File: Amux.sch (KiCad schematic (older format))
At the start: 3 parts, among them U16 74LVC32, U6 74LVC257, U7 74LVC257

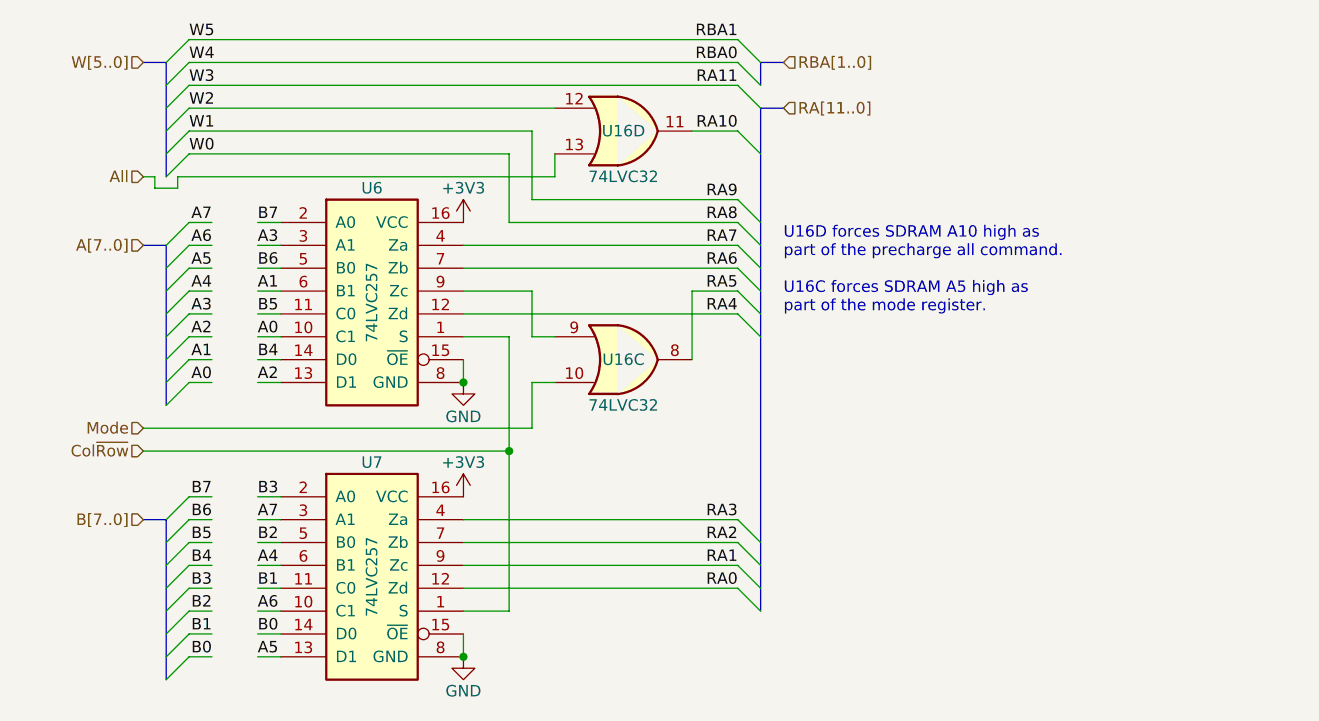
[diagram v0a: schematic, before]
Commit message: PAL
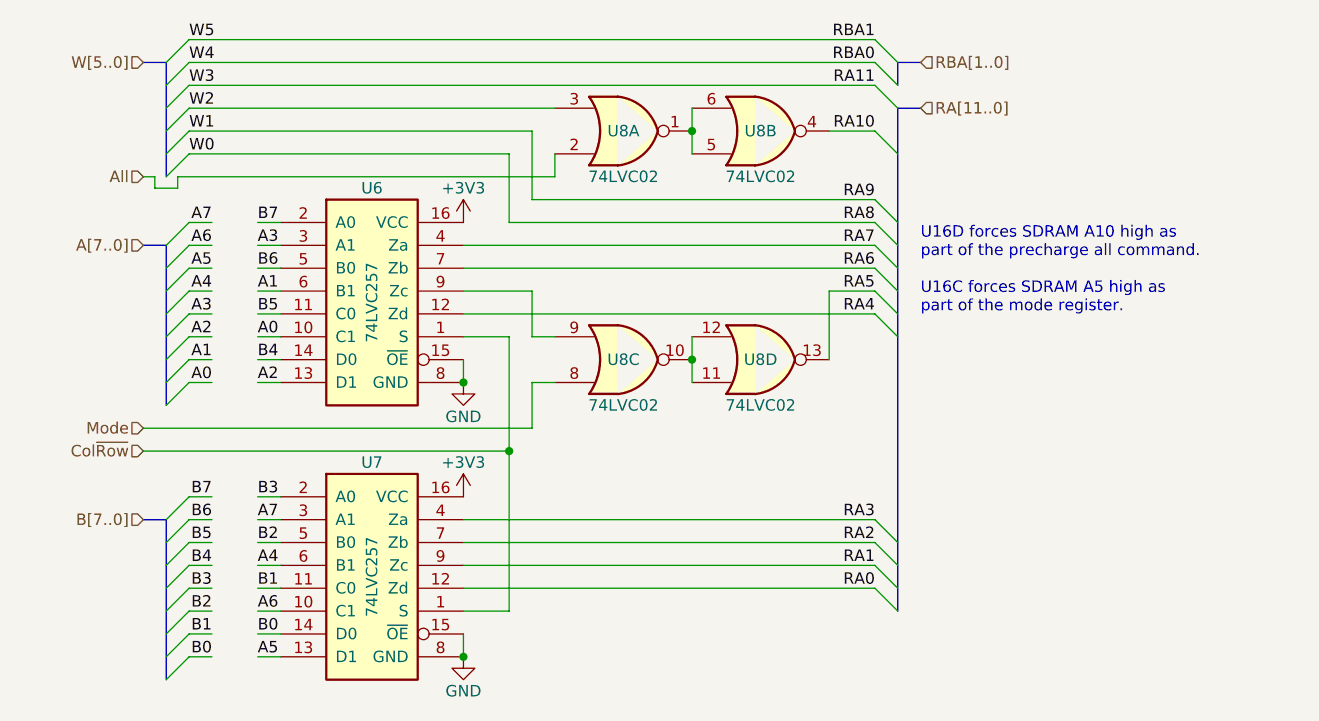
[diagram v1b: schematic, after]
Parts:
- removed U16: 74LVC32, stdpads:TSSOP-14_4.4x5mm_P0.65mm, symbol 74xx:74LS32
- added U8: 74LVC02, stdpads:TSSOP-14_4.4x5mm_P0.65mm, symbol 74xx:74LS02
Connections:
- net All: now also U8.2
- net Mode: now also U8.8
- net RA10: now also U8.4
- net RA5: now also U8.13
- net W2: now also U8.3
- net at U6.9 (Zc): now also U8.9
- new net: U8.10, U8.11, U8.12
- new net: U8.1, U8.5, U8.6
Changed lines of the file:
@@
 $Descr USLetter 11000 8500
 encoding utf-8
-Sheet 6 6
+Sheet 3 5
 Title ""
 Date ""
@@
 $EndComp
 Connection ~ 5500 5450
-Text Label 6700 5150 2    50   ~ 0
-RA0
-Text Label 6700 5050 2    50   ~ 0
-RA1
-Text Label 6700 4950 2    50   ~ 0
-RA2
-Text Label 6700 4850 2    50   ~ 0
-RA3
 Text Label 4600 4050 0    50   ~ 0
 A0
@@
 Text Label 4600 4850 0    50   ~ 0
 A7
-Text Label 6700 3650 2    50   ~ 0
-RA7
-Text Label 6700 3750 2    50   ~ 0
-RA6
-Text Label 6700 3950 2    50   ~ 0
-RA4
 Text Label 4600 5350 0    50   ~ 0
 B0
@@
 Text Label 4600 3550 0    50   ~ 0
 B7
-Text Label 6700 3550 2    50   ~ 0
-RA8
-Text Label 6700 3450 2    50   ~ 0
-RA9
 Text Label 4300 3250 0    50   ~ 0
 W0
 Text Label 4300 3150 0    50   ~ 0
 W1
-Text Label 6700 3150 2    50   ~ 0
-RA10
-Text Label 6700 2950 2    50   ~ 0
-RA11
 Text Label 4300 3050 0    50   ~ 0
 W2
 Text Label 4300 2950 0    50   ~ 0
 W3
-Text Label 6700 2850 2    50   ~ 0
-RBA0
 Text Label 4300 2850 0    50   ~ 0
 W4
@@
 Wire Wire Line
 	5700 4550 5700 5250
-Wire Wire Line
-	6700 5150 5500 5150
-Wire Wire Line
-	5500 5050 6700 5050
-Wire Wire Line
-	6700 4950 5500 4950
-Wire Wire Line
-	5500 4850 6700 4850
-Wire Wire Line
-	6700 3950 5500 3950
-Wire Wire Line
-	5500 3750 6700 3750
-$Comp
-L 74xx:74LS32 U?
-U 4 1 6061EDB0
-P 6200 3150
-AR Path="/CF1C1573/6061EDB0" Ref="U?"  Part="1"
-AR Path="/6061EDB0" Ref="U?"  Part="1"
-AR Path="/6060D166/6061EDB0" Ref="U16"  Part="4"
-F 0 "U16" H 6200 3150 50  0000 C CNN
-F 1 "74LVC32" H 6200 2950 50  0000 C CNN
-F 2 "stdpads:TSSOP-14_4.4x5mm_P0.65mm" H 6200 3150 50  0001 C CNN
-F 3 "http://www.ti.com/lit/gpn/sn74ls02" H 6200 3150 50  0001 C CNN
-	4    6200 3150
-	1    0    0    -1
-$EndComp
-Wire Wire Line
-	5700 3550 6700 3550
-Wire Wire Line
-	6700 3450 5800 3450
 Wire Wire Line
 	5700 3250 5700 3550
@@
 	1    0    0    -1
 $EndComp
-Wire Wire Line
-	5500 3650 6700 3650
-Wire Wire Line
-	6700 3150 6500 3150
-Wire Wire Line
-	6700 3850 6500 3850
-$Comp
-L 74xx:74LS32 U?
-U 3 1 6061EDE7
-P 6200 4150
-AR Path="/CF1C1573/6061EDE7" Ref="U?"  Part="1"
-AR Path="/6061EDE7" Ref="U?"  Part="1"
-AR Path="/6060D166/6061EDE7" Ref="U16"  Part="3"
-F 0 "U16" H 6200 4150 50  0000 C CNN
-F 1 "74LVC32" H 6200 3950 50  0000 C CNN
-F 2 "stdpads:TSSOP-14_4.4x5mm_P0.65mm" H 6200 4150 50  0001 C CNN
-F 3 "http://www.ti.com/lit/gpn/sn74ls02" H 6200 4150 50  0001 C CNN
-	3    6200 4150
-	1    0    0    -1
-$EndComp
-Wire Wire Line
-	6500 3850 6500 4150
-Text Label 6700 2750 2    50   ~ 0
-RBA1
 Text HLabel 4100 2850 0    50   Input ~ 0
 W[5..0]
@@
 	4100 2850 4200 2850
 Wire Wire Line
-	4300 2750 6700 2750
-Wire Wire Line
-	4300 2850 6700 2850
-Wire Wire Line
-	4300 2950 6700 2950
+	4300 2750 7300 2750
+Wire Wire Line
+	4300 2850 7300 2850
 Wire Wire Line
 	4300 3050 5900 3050
@@
 Wire Wire Line
 	4250 3350 5900 3350
-Text HLabel 6900 2850 2    50   Input ~ 0
+Text HLabel 7500 2850 2    50   Input ~ 0
 RBA[1..0]
 Entry Wire Line
-	6800 2950 6700 2850
-Entry Wire Line
-	6800 2850 6700 2750
-Wire Bus Line
-	6900 2850 6800 2850
-Wire Bus Line
-	6800 2850 6800 2950
-Entry Wire Line
-	6800 3250 6700 3150
-Entry Wire Line
-	6800 3050 6700 2950
-Wire Bus Line
-	6900 3050 6800 3050
-Text HLabel 6900 3050 2    50   Input ~ 0
+	7400 2950 7300 2850
+Entry Wire Line
+	7400 2850 7300 2750
+Wire Bus Line
+	7500 2850 7400 2850
+Wire Bus Line
+	7400 2850 7400 2950
+Wire Bus Line
+	7500 3050 7400 3050
+Text HLabel 7500 3050 2    50   Input ~ 0
 RA[11..0]
-Entry Wire Line
-	6800 3650 6700 3550
-Entry Wire Line
-	6800 3550 6700 3450
-Entry Wire Line
-	6800 3750 6700 3650
-Entry Wire Line
-	6800 3950 6700 3850
-Entry Wire Line
-	6800 3850 6700 3750
-Entry Wire Line
-	6800 4050 6700 3950
-Entry Wire Line
-	6800 5050 6700 4950
-Entry Wire Line
-	6800 4950 6700 4850
-Entry Wire Line
-	6800 5150 6700 5050
-Entry Wire Line
-	6800 5250 6700 5150
 Wire Wire Line
 	4250 3400 4250 3350
@@
 Wire Wire Line
 	5800 4250 5800 4450
-Text Notes 6900 3950 0    50   ~ 0
+Text Notes 7500 3950 0    50   ~ 0
 U16D forces SDRAM A10 high as\npart of the precharge all command.\n\nU16C forces SDRAM A5 high as\npart of the mode register.
-Text Label 6700 3850 2    50   ~ 0
+Wire Wire Line
+	7300 5150 5500 5150
+Wire Wire Line
+	5500 5050 7300 5050
+Wire Wire Line
+	5500 4850 7300 4850
+Wire Wire Line
+	7300 4950 5500 4950
+Wire Wire Line
+	7300 3950 5500 3950
+Wire Wire Line
+	5500 3750 7300 3750
+Wire Wire Line
+	7300 3850 7100 3850
+Wire Wire Line
+	5500 3650 7300 3650
+Wire Wire Line
+	7300 3450 5800 3450
+Wire Wire Line
+	5700 3550 7300 3550
+Wire Wire Line
+	4300 2950 7300 2950
+Entry Wire Line
+	7400 5250 7300 5150
+Entry Wire Line
+	7400 5150 7300 5050
+Entry Wire Line
+	7400 4950 7300 4850
+Entry Wire Line
+	7400 5050 7300 4950
+Entry Wire Line
+	7400 4050 7300 3950
+Entry Wire Line
+	7400 3850 7300 3750
+Entry Wire Line
+	7400 3950 7300 3850
+Entry Wire Line
+	7400 3750 7300 3650
+Entry Wire Line
+	7400 3550 7300 3450
+Entry Wire Line
+	7400 3650 7300 3550
+Entry Wire Line
+	7400 3050 7300 2950
+Entry Wire Line
+	7400 3250 7300 3150
+Text Label 7300 3850 2    50   ~ 0
 RA5
+Text Label 7300 2750 2    50   ~ 0
+RBA1
+Text Label 7300 2850 2    50   ~ 0
+RBA0
+Text Label 7300 2950 2    50   ~ 0
+RA11
+Text Label 7300 3150 2    50   ~ 0
+RA10
+Text Label 7300 3450 2    50   ~ 0
+RA9
+Text Label 7300 3550 2    50   ~ 0
+RA8
+Text Label 7300 3950 2    50   ~ 0
+RA4
+Text Label 7300 3750 2    50   ~ 0
+RA6
+Text Label 7300 3650 2    50   ~ 0
+RA7
+Text Label 7300 4850 2    50   ~ 0
+RA3
+Text Label 7300 4950 2    50   ~ 0
+RA2
+Text Label 7300 5050 2    50   ~ 0
+RA1
+Text Label 7300 5150 2    50   ~ 0
+RA0
+$Comp
+L 74xx:74LS02 U?
+U 3 1 64E55E47
+P 6200 4150
+AR Path="/606ED367/64E55E47" Ref="U?"  Part="1"
+AR Path="/64E55E47" Ref="U?"  Part="1"
+AR Path="/6060D166/64E55E47" Ref="U8"  Part="3"
+F 0 "U8" H 6200 4150 50  0000 C CNN
+F 1 "74LVC02" H 6200 4350 50  0000 C CNN
+F 2 "stdpads:TSSOP-14_4.4x5mm_P0.65mm" H 6200 4150 50  0001 C CNN
+F 3 "http://www.ti.com/lit/gpn/sn74LS08" H 6200 4150 50  0001 C CNN
+	3    6200 4150
+	1    0    0    1
+$EndComp
+$Comp
+L 74xx:74LS02 U?
+U 4 1 64E60EEF
+P 6800 4150
+AR Path="/606ED367/64E60EEF" Ref="U?"  Part="1"
+AR Path="/64E60EEF" Ref="U?"  Part="1"
+AR Path="/6060D166/64E60EEF" Ref="U8"  Part="4"
+F 0 "U8" H 6800 4150 50  0000 C CNN
+F 1 "74LVC02" H 6800 4350 50  0000 C CNN
+F 2 "stdpads:TSSOP-14_4.4x5mm_P0.65mm" H 6800 4150 50  0001 C CNN
+F 3 "http://www.ti.com/lit/gpn/sn74LS08" H 6800 4150 50  0001 C CNN
+	4    6800 4150
+	1    0    0    1
+$EndComp
+Wire Wire Line
+	7100 4150 7100 3850
+Wire Wire Line
+	6500 4050 6500 4150
+Connection ~ 6500 4150
+Wire Wire Line
+	6500 4150 6500 4250
+$Comp
+L 74xx:74LS02 U?
+U 1 1 64E69A1A
+P 6200 3150
+AR Path="/606ED367/64E69A1A" Ref="U?"  Part="1"
+AR Path="/64E69A1A" Ref="U?"  Part="1"
+AR Path="/6060D166/64E69A1A" Ref="U8"  Part="1"
+F 0 "U8" H 6200 3150 50  0000 C CNN
+F 1 "74LVC02" H 6200 3350 50  0000 C CNN
+F 2 "stdpads:TSSOP-14_4.4x5mm_P0.65mm" H 6200 3150 50  0001 C CNN
+F 3 "http://www.ti.com/lit/gpn/sn74LS08" H 6200 3150 50  0001 C CNN
+	1    6200 3150
+	1    0    0    1
+$EndComp
+$Comp
+L 74xx:74LS02 U?
+U 2 1 64E6CFE8
+P 6800 3150
+AR Path="/606ED367/64E6CFE8" Ref="U?"  Part="1"
+AR Path="/64E6CFE8" Ref="U?"  Part="1"
+AR Path="/6060D166/64E6CFE8" Ref="U8"  Part="2"
+F 0 "U8" H 6800 3150 50  0000 C CNN
+F 1 "74LVC02" H 6800 3350 50  0000 C CNN
+F 2 "stdpads:TSSOP-14_4.4x5mm_P0.65mm" H 6800 3150 50  0001 C CNN
+F 3 "http://www.ti.com/lit/gpn/sn74LS08" H 6800 3150 50  0001 C CNN
+	2    6800 3150
+	1    0    0    1
+$EndComp
+Wire Wire Line
+	7300 3150 7100 3150
+Wire Wire Line
+	6500 3050 6500 3150
 Wire Bus Line
 	4200 2850 4200 3350
@@
 	4200 3650 4200 4350
 Wire Bus Line
-	6800 3050 6800 5250
+	7400 3050 7400 5250
+Connection ~ 6500 3150
+Wire Wire Line
+	6500 3150 6500 3250
 $EndSCHEMATC
